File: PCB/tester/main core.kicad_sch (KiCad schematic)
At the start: 44 parts, among them J2 PR20203VBDN, Q1 DMN63D8L-7, SW1 TL3305BF260QG, SW2 TL3305BF260QG, SW3 TL3305BF260QG, SW4 TL3305BF260QG, SW5 TL3305BF260QG, SW6 TL3305BF260QG, SW7 TL3305BF260QG, SW8 TL3305BF260QG, SW9 TL3305BF260QG, U5 ATXMEGA32A4U-MH

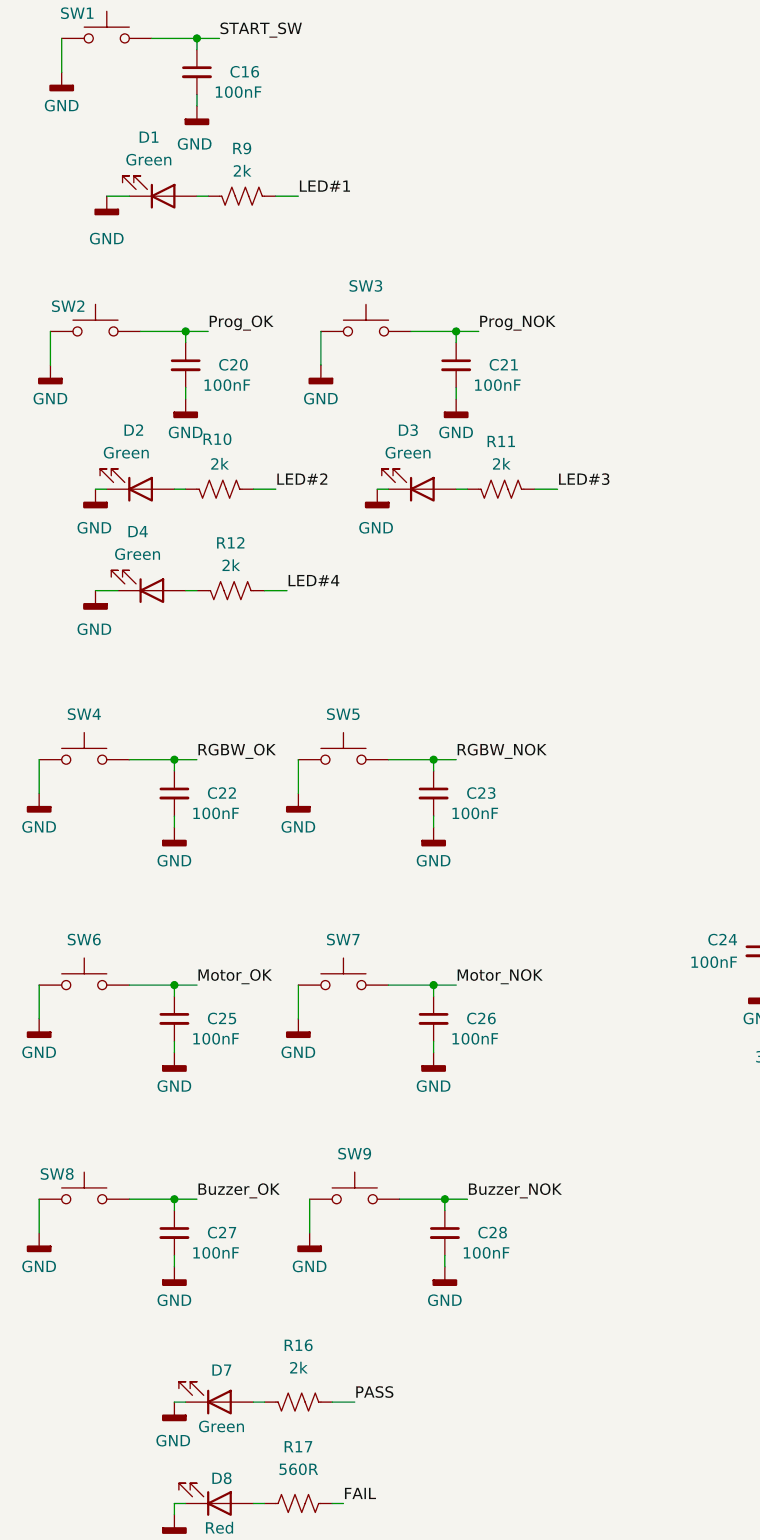
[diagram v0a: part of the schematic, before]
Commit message: sync with main
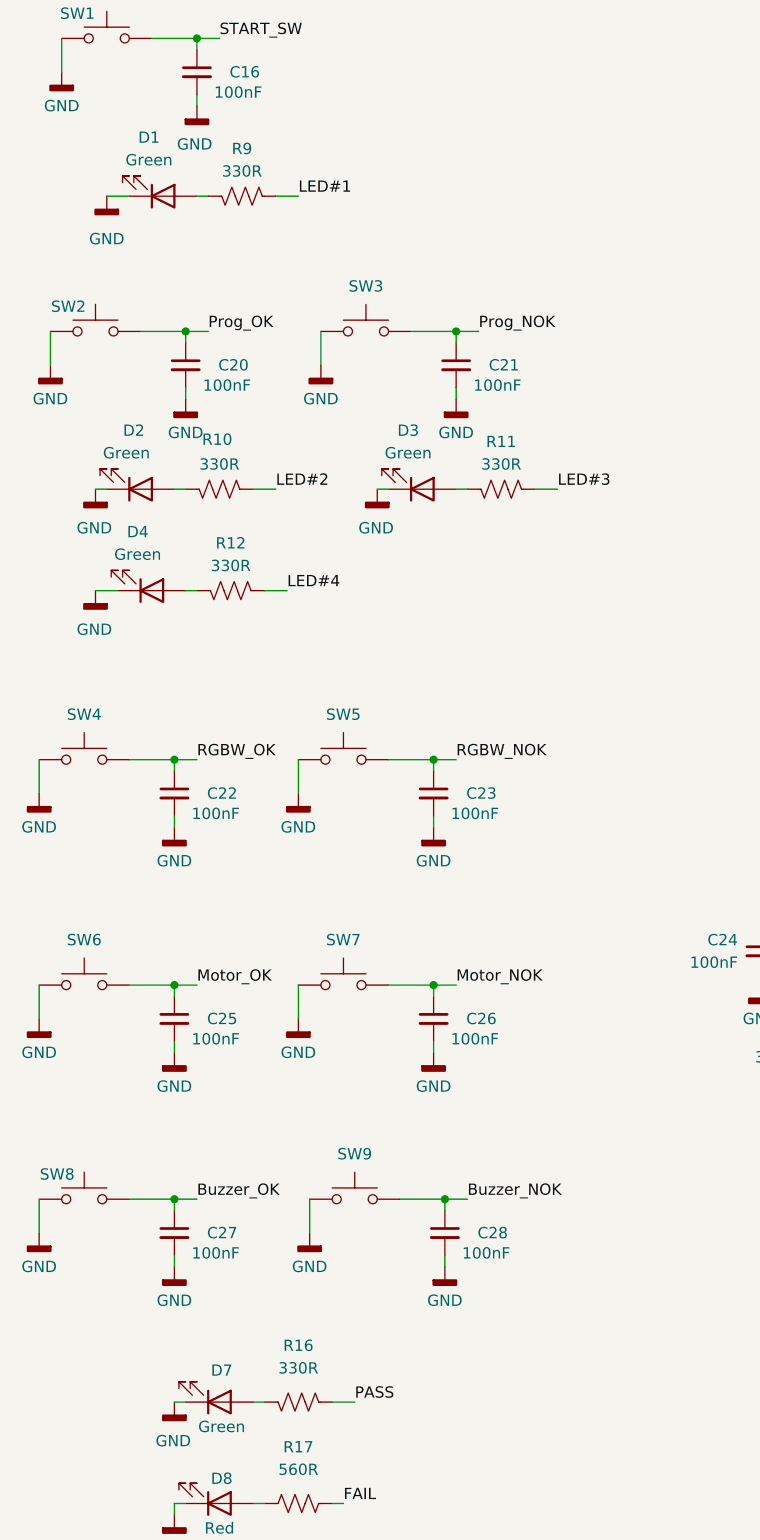
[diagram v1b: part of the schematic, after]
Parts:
- R10, R11, R12, R16, R9: value 2k -> 330R; MPN ERJ-2RKF2001X -> CRCW0402330RFKEDHP; OEPSPN OEPS020007 -> OEPS020191
